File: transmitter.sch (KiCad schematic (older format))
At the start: 34 parts, among them J10 Conn_Coaxial, J9 Conn_Coaxial, U22 LM321, U23 HMC430, U24 RFPA5542

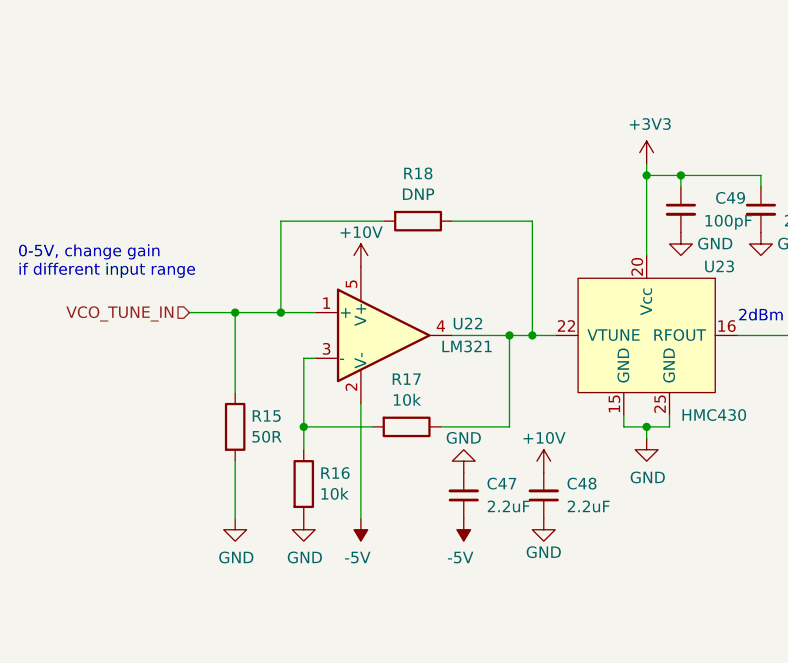
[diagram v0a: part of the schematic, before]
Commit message: Added connector
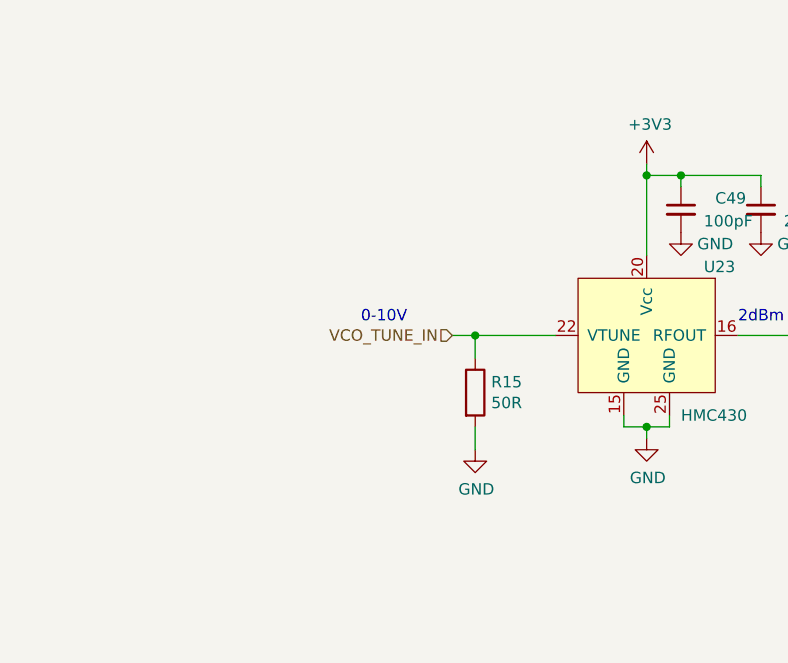
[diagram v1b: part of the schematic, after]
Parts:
- removed C47, C48: 2.2uF, Capacitor_SMD:C_0603_1608Metric_Pad1.08x0.95mm_HandSolder, symbol Device:C_Small
- removed R16, R17: 10k, Resistor_SMD:R_0603_1608Metric_Pad0.98x0.95mm_HandSolder, symbol Device:R
- removed R18: DNP, Resistor_SMD:R_0603_1608Metric_Pad0.98x0.95mm_HandSolder, symbol Device:R
- removed U22: LM321, Package_TO_SOT_SMD:SOT-23-5, symbol Amplifier_Operational:LM321
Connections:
- net VCO_TUNE_IN: now also U23.22 (VTUNE)
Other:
- note added: "0-10V"
- note removed: "0-5V, change gain\nif different input range"
- moved on the sheet: R15
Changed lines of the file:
@@
 	1    0    0    -1
 $EndComp
-Text HLabel 2150 3750 0    50   Input ~ 0
+Text HLabel 3300 3850 0    50   Input ~ 0
 VCO_TUNE_IN
 $Comp
@@
 Wire Wire Line
 	8700 4600 10000 4600
-Text Notes 1400 3600 0    50   ~ 0
-0-5V, change gain\nif different input range
-$Comp
-L power:+10V #PWR075
-U 1 1 5FB646C4
-P 2900 3550
-F 0 "#PWR075" H 2900 3400 50  0001 C CNN
-F 1 "+10V" H 2900 3700 50  0000 C CNN
-F 2 "" H 2900 3550 50  0001 C CNN
-F 3 "" H 2900 3550 50  0001 C CNN
-	1    2900 3550
-	1    0    0    -1
-$EndComp
-$Comp
-L Device:R R16
-U 1 1 5FB6992C
-P 2650 4500
-F 0 "R16" H 2720 4546 50  0000 L CNN
-F 1 "10k" H 2720 4455 50  0000 L CNN
-F 2 "Resistor_SMD:R_0603_1608Metric_Pad0.98x0.95mm_HandSolder" V 2580 4500 50  0001 C CNN
-F 3 "~" H 2650 4500 50  0001 C CNN
-	1    2650 4500
-	1    0    0    -1
-$EndComp
-$Comp
-L power:GND #PWR074
-U 1 1 5FB6A38F
-P 2650 4650
-F 0 "#PWR074" H 2650 4400 50  0001 C CNN
-F 1 "GND" H 2655 4477 50  0000 C CNN
-F 2 "" H 2650 4650 50  0001 C CNN
-F 3 "" H 2650 4650 50  0001 C CNN
-	1    2650 4650
-	1    0    0    -1
-$EndComp
-Wire Wire Line
-	2650 4350 2650 4250
-Wire Wire Line
-	2650 4250 2650 3950
-Wire Wire Line
-	2650 3950 2700 3950
-Connection ~ 2650 4250
-Wire Wire Line
-	3300 3850 3550 3850
-Wire Wire Line
-	3550 4250 3550 3850
-Connection ~ 3550 3850
-Wire Wire Line
-	2650 4250 2950 4250
-$Comp
-L Device:R R18
-U 1 1 5FB809BA
-P 3150 3350
-F 0 "R18" V 2943 3350 50  0000 C CNN
-F 1 "DNP" V 3034 3350 50  0000 C CNN
-F 2 "Resistor_SMD:R_0603_1608Metric_Pad0.98x0.95mm_HandSolder" V 3080 3350 50  0001 C CNN
-F 3 "~" H 3150 3350 50  0001 C CNN
-	1    3150 3350
-	0    1    1    0
-$EndComp
-Wire Wire Line
-	2550 3750 2550 3350
-Wire Wire Line
-	2550 3350 3000 3350
-Connection ~ 2550 3750
-Wire Wire Line
-	2550 3750 2700 3750
-Wire Wire Line
-	3300 3350 3650 3350
-Wire Wire Line
-	3250 4250 3550 4250
-$Comp
-L Device:R R17
-U 1 1 5FB68EC6
-P 3100 4250
-F 0 "R17" V 2893 4250 50  0000 C CNN
-F 1 "10k" V 2984 4250 50  0000 C CNN
-F 2 "Resistor_SMD:R_0603_1608Metric_Pad0.98x0.95mm_HandSolder" V 3030 4250 50  0001 C CNN
-F 3 "~" H 3100 4250 50  0001 C CNN
-	1    3100 4250
-	0    1    1    0
-$EndComp
-Wire Wire Line
-	3550 3850 3650 3850
-Wire Wire Line
-	3650 3850 3650 3350
-Connection ~ 3650 3850
-Wire Wire Line
-	3650 3850 3750 3850
+Text Notes 2900 3800 0    50   ~ 0
+0-10V
 Wire Wire Line
 	7750 3850 8250 3850
@@
 	5800 3300 5800 3350
 $Comp
-L Device:C_Small C48
-U 1 1 5FBEA831
-P 3700 4550
-F 0 "C48" H 3800 4500 50  0000 L CNN
-F 1 "2.2uF" H 3800 4600 50  0000 L CNN
-F 2 "Capacitor_SMD:C_0603_1608Metric_Pad1.08x0.95mm_HandSolder" H 3700 4550 50  0001 C CNN
-F 3 "~" H 3700 4550 50  0001 C CNN
-	1    3700 4550
-	1    0    0    1
-$EndComp
-$Comp
-L power:GND #PWR080
-U 1 1 5FBEA837
-P 3700 4650
-F 0 "#PWR080" H 3700 4400 50  0001 C CNN
-F 1 "GND" H 3700 4500 50  0000 C CNN
-F 2 "" H 3700 4650 50  0001 C CNN
-F 3 "" H 3700 4650 50  0001 C CNN
-	1    3700 4650
-	-1   0    0    -1
-$EndComp
-Wire Wire Line
-	2150 3750 2350 3750
-$Comp
 L Device:R R15
 U 1 1 605E2B48
-P 2350 4250
-F 0 "R15" H 2420 4296 50  0000 L CNN
-F 1 "50R" H 2420 4205 50  0000 L CNN
-F 2 "Resistor_SMD:R_0603_1608Metric_Pad0.98x0.95mm_HandSolder" V 2280 4250 50  0001 C CNN
-F 3 "~" H 2350 4250 50  0001 C CNN
-	1    2350 4250
+P 3400 4100
+F 0 "R15" H 3470 4146 50  0000 L CNN
+F 1 "50R" H 3470 4055 50  0000 L CNN
+F 2 "Resistor_SMD:R_0603_1608Metric_Pad0.98x0.95mm_HandSolder" V 3330 4100 50  0001 C CNN
+F 3 "~" H 3400 4100 50  0001 C CNN
+	1    3400 4100
 	1    0    0    -1
 $EndComp
@@
 L power:GND #PWR073
 U 1 1 605E6DB6
-P 2350 4650
-F 0 "#PWR073" H 2350 4400 50  0001 C CNN
-F 1 "GND" H 2355 4477 50  0000 C CNN
-F 2 "" H 2350 4650 50  0001 C CNN
-F 3 "" H 2350 4650 50  0001 C CNN
-	1    2350 4650
-	1    0    0    -1
-$EndComp
-Wire Wire Line
-	2350 4650 2350 4400
-Wire Wire Line
-	2350 4100 2350 3750
-Connection ~ 2350 3750
-Wire Wire Line
-	2350 3750 2550 3750
-$Comp
-L Amplifier_Operational:LM321 U22
-U 1 1 605F5A8B
-P 3000 3850
-F 0 "U22" H 3300 3900 50  0000 L CNN
-F 1 "LM321" H 3250 3800 50  0000 L CNN
-F 2 "Package_TO_SOT_SMD:SOT-23-5" H 3000 3850 50  0001 C CNN
-F 3 "http://www.ti.com/lit/ds/symlink/lm321.pdf" H 3000 3850 50  0001 C CNN
-	1    3000 3850
-	1    0    0    -1
-$EndComp
-Wire Wire Line
-	2900 4650 2900 4150
-$Comp
-L power:+10V #PWR079
-U 1 1 6060A82F
-P 3700 4450
-F 0 "#PWR079" H 3700 4300 50  0001 C CNN
-F 1 "+10V" H 3700 4600 50  0000 C CNN
-F 2 "" H 3700 4450 50  0001 C CNN
-F 3 "" H 3700 4450 50  0001 C CNN
-	1    3700 4450
-	1    0    0    -1
-$EndComp
-$Comp
-L power:-5V #PWR076
-U 1 1 60622B56
-P 2900 4650
-F 0 "#PWR076" H 2900 4750 50  0001 C CNN
-F 1 "-5V" H 2915 4823 50  0000 C CNN
-F 2 "" H 2900 4650 50  0001 C CNN
-F 3 "" H 2900 4650 50  0001 C CNN
-	1    2900 4650
-	-1   0    0    1
-$EndComp
+P 3400 4350
+F 0 "#PWR073" H 3400 4100 50  0001 C CNN
+F 1 "GND" H 3405 4177 50  0000 C CNN
+F 2 "" H 3400 4350 50  0001 C CNN
+F 3 "" H 3400 4350 50  0001 C CNN
+	1    3400 4350
+	1    0    0    -1
+$EndComp
+Wire Wire Line
+	3400 4350 3400 4250
+Wire Wire Line
+	3400 3950 3400 3850
 Wire Wire Line
 	7400 4050 7700 4050
@@
 Wire Wire Line
 	8250 3850 8250 3950
-$Comp
-L Device:C_Small C47
-U 1 1 606D688F
-P 3350 4550
-F 0 "C47" H 3450 4500 50  0000 L CNN
-F 1 "2.2uF" H 3450 4600 50  0000 L CNN
-F 2 "Capacitor_SMD:C_0603_1608Metric_Pad1.08x0.95mm_HandSolder" H 3350 4550 50  0001 C CNN
-F 3 "~" H 3350 4550 50  0001 C CNN
-	1    3350 4550
-	1    0    0    1
-$EndComp
-$Comp
-L power:GND #PWR077
-U 1 1 606D6895
-P 3350 4450
-F 0 "#PWR077" H 3350 4200 50  0001 C CNN
-F 1 "GND" H 3350 4300 50  0000 C CNN
-F 2 "" H 3350 4450 50  0001 C CNN
-F 3 "" H 3350 4450 50  0001 C CNN
-	1    3350 4450
-	1    0    0    1
-$EndComp
-$Comp
-L power:-5V #PWR078
-U 1 1 606DB6B0
-P 3350 4650
-F 0 "#PWR078" H 3350 4750 50  0001 C CNN
-F 1 "-5V" H 3365 4823 50  0000 C CNN
-F 2 "" H 3350 4650 50  0001 C CNN
-F 3 "" H 3350 4650 50  0001 C CNN
-	1    3350 4650
-	-1   0    0    1
-$EndComp
 Wire Wire Line
 	5500 4750 5600 4750
+Wire Wire Line
+	3300 3850 3400 3850
+Wire Wire Line
+	3750 3850 3400 3850
+Connection ~ 3400 3850
 $EndSCHEMATC

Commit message: First layout
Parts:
- J10, J9: footprint (none) -> Connector_Coaxial:SMA_Amphenol_901-144_Vertical
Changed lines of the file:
@@
 F 0 "J10" V 8250 4550 50  0000 L CNN
 F 1 "Conn_Coaxial" V 8350 4300 50  0000 L CNN
-F 2 "" H 8250 4400 50  0001 C CNN
+F 2 "Connector_Coaxial:SMA_Amphenol_901-144_Vertical" H 8250 4400 50  0001 C CNN
 F 3 " ~" H 8250 4400 50  0001 C CNN
 	1    8250 4400
@@
 F 0 "J9" V 5750 3250 50  0000 L CNN
 F 1 "Conn_Coaxial" V 5650 3050 50  0000 L CNN
-F 2 "" H 5550 3300 50  0001 C CNN
+F 2 "Connector_Coaxial:SMA_Amphenol_901-144_Vertical" H 5550 3300 50  0001 C CNN
 F 3 " ~" H 5550 3300 50  0001 C CNN
 	1    5550 3300

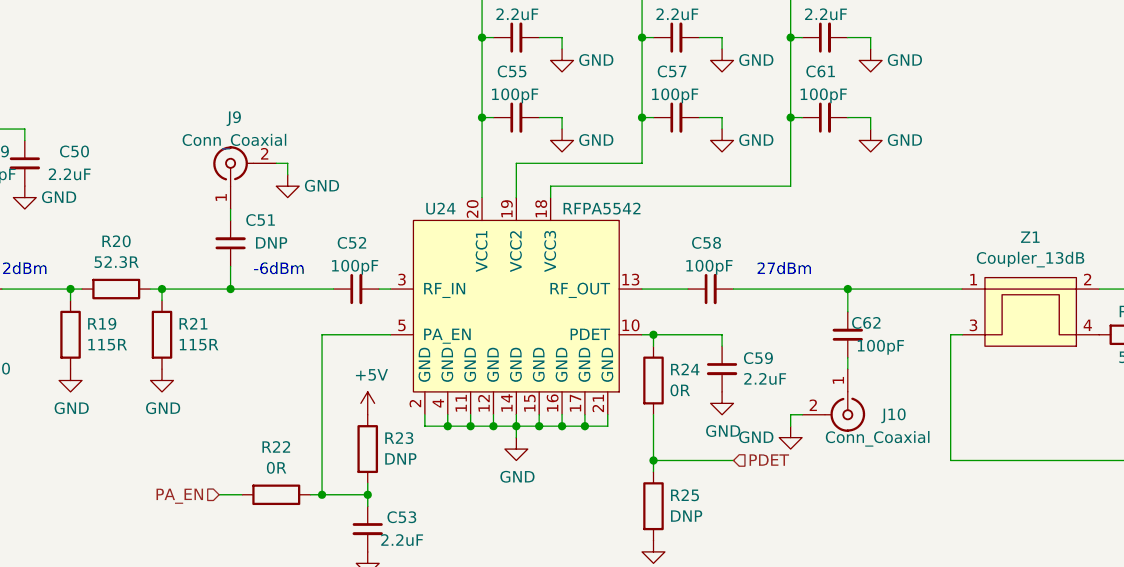
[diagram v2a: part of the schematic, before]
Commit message: Curved tracks
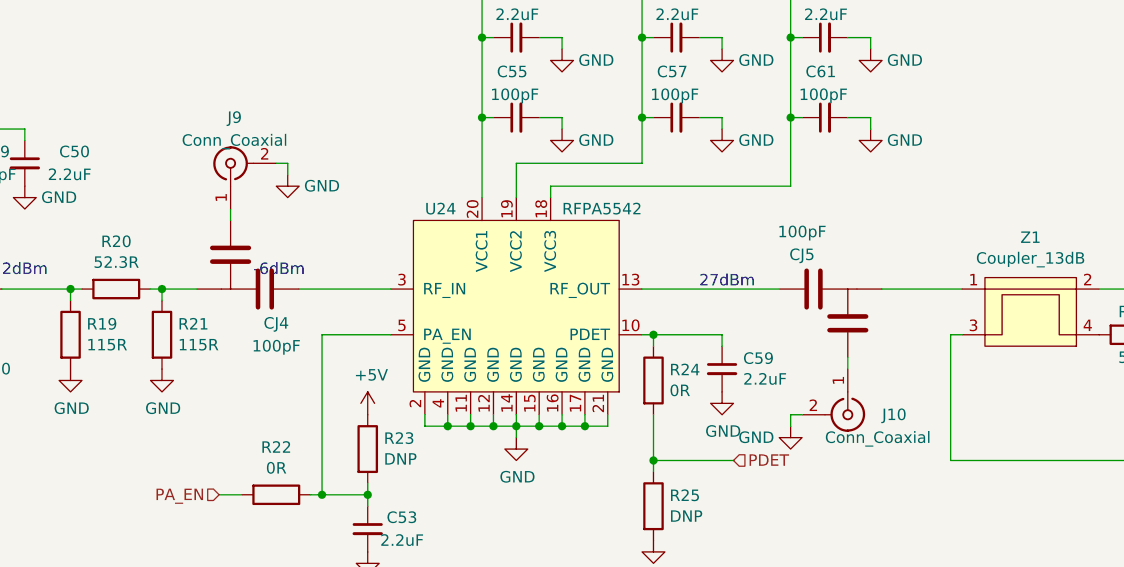
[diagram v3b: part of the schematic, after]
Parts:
- removed C51: DNP, Capacitor_SMD:C_0402_1005Metric, symbol Device:C_Small
- removed C52, C58, C62: 100pF, Capacitor_SMD:C_0402_1005Metric, symbol Device:C_Small
- added CJ4, CJ5: 100pF, own:0402_Jumper_Tapered, symbol own:C_Jumper
- R26: footprint Resistor_SMD:R_0402_1005Metric -> own:0402_Tapered
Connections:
- net at U24.13 (RF_OUT): now also CJ5.2
- net at Z1.1: now also CJ5.1
- net at U24.3 (RF_IN): now also CJ4.2
- net at R20.1, R21.1: now also CJ4.1
- net at J10.1 (In): now also CJ5.3
- net at J9.1 (In): now also CJ4.3
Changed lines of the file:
@@
 F 0 "R26" V 9400 4050 50  0000 C CNN
 F 1 "50R" V 9600 4050 50  0000 C CNN
-F 2 "Resistor_SMD:R_0402_1005Metric" V 9430 4050 50  0001 C CNN
+F 2 "own:0402_Tapered" V 9430 4050 50  0001 C CNN
 F 3 "~" H 9500 4050 50  0001 C CNN
 	1    9500 4050
@@
 Wire Wire Line
 	9700 4050 9650 4050
-$Comp
-L Device:C_Small C58
-U 1 1 5FAEA3FD
-P 7650 3850
-F 0 "C58" V 7850 3800 50  0000 L CNN
-F 1 "100pF" V 7750 3750 50  0000 L CNN
-F 2 "Capacitor_SMD:C_0402_1005Metric" H 7650 3850 50  0001 C CNN
-F 3 "~" H 7650 3850 50  0001 C CNN
-	1    7650 3850
-	0    -1   -1   0
-$EndComp
-Wire Wire Line
-	7350 3850 7550 3850
 Text HLabel 10000 3850 2    50   Input ~ 0
 RF_OUT
@@
 Text HLabel 5500 4750 0    50   Input ~ 0
 PA_EN
-$Comp
-L Device:C_Small C52
-U 1 1 5FB18027
-P 6100 3850
-F 0 "C52" V 6300 3800 50  0000 L CNN
-F 1 "100pF" V 6200 3750 50  0000 L CNN
-F 2 "Capacitor_SMD:C_0402_1005Metric" H 6100 3850 50  0001 C CNN
-F 3 "~" H 6100 3850 50  0001 C CNN
-	1    6100 3850
-	0    -1   -1   0
-$EndComp
-Wire Wire Line
-	6200 3850 6250 3850
-Text Notes 7850 3800 0    50   ~ 0
+Text Notes 7600 3850 0    50   ~ 0
 27dBm
 Text Notes 9500 3800 0    50   ~ 0
@@
 Wire Wire Line
 	5250 3900 5250 3850
-Connection ~ 5250 3850
 $Comp
 L power:GND #PWR086
@@
 Text Notes 2900 3800 0    50   ~ 0
 0-10V
-Wire Wire Line
-	7750 3850 8250 3850
 $Comp
 L Connector:Conn_Coaxial J10
@@
 	0    1    1    0
 $EndComp
-Connection ~ 8250 3850
-Wire Wire Line
-	8250 3850 8750 3850
 $Comp
 L power:GND #PWR0100
@@
 	4850 3850 4550 3850
 Connection ~ 4850 3850
-Wire Wire Line
-	5250 3850 5550 3850
 $Comp
 L Connector:Conn_Coaxial J9
@@
 Wire Wire Line
 	5800 3300 5750 3300
-Connection ~ 5550 3850
-Wire Wire Line
-	5550 3850 6000 3850
 Wire Wire Line
 	5800 3300 5800 3350
@@
 	7400 4050 7700 4050
 Connection ~ 7400 4050
-$Comp
-L Device:C_Small C51
-U 1 1 6063F390
-P 5550 3650
-F 0 "C51" H 5350 3550 50  0000 L CNN
-F 1 "DNP" H 5300 3650 50  0000 L CNN
-F 2 "Capacitor_SMD:C_0402_1005Metric" H 5550 3650 50  0001 C CNN
-F 3 "~" H 5550 3650 50  0001 C CNN
-	1    5550 3650
-	-1   0    0    1
-$EndComp
 Wire Wire Line
 	5550 3550 5550 3500
 Wire Wire Line
-	5550 3750 5550 3850
-$Comp
-L Device:C_Small C62
-U 1 1 6064CE61
-P 8250 4050
-F 0 "C62" H 8100 4000 50  0000 L CNN
-F 1 "100pF" H 8000 4100 50  0000 L CNN
-F 2 "Capacitor_SMD:C_0402_1005Metric" H 8250 4050 50  0001 C CNN
-F 3 "~" H 8250 4050 50  0001 C CNN
-	1    8250 4050
-	-1   0    0    1
-$EndComp
-Wire Wire Line
 	8250 4150 8250 4200
-Wire Wire Line
-	8250 3850 8250 3950
 Wire Wire Line
 	5500 4750 5600 4750
@@
 	3750 3850 3400 3850
 Connection ~ 3400 3850
+$Comp
+L own:C_Jumper CJ4
+U 1 1 606BB88C
+P 5550 3700
+F 0 "CJ4" H 5750 3400 50  0000 C CNN
+F 1 "100pF" H 5750 3300 50  0000 C CNN
+F 2 "own:0402_Jumper_Tapered" H 5588 3550 50  0001 C CNN
+F 3 "~" H 5550 3700 50  0001 C CNN
+	1    5550 3700
+	1    0    0    -1
+$EndComp
+Wire Wire Line
+	5250 3850 5400 3850
+Connection ~ 5250 3850
+Wire Wire Line
+	5850 3850 6250 3850
+$Comp
+L own:C_Jumper CJ5
+U 1 1 606CBCB9
+P 8250 4000
+F 0 "CJ5" H 8450 3700 50  0000 C CNN
+F 1 "100pF" H 8450 3600 50  0000 C CNN
+F 2 "own:0402_Jumper_Tapered" H 8288 3850 50  0001 C CNN
+F 3 "~" H 8250 4000 50  0001 C CNN
+	1    8250 4000
+	-1   0    0    1
+$EndComp
+Wire Wire Line
+	7950 3850 7350 3850
+Wire Wire Line
+	8400 3850 8750 3850
 $EndSCHEMATC
